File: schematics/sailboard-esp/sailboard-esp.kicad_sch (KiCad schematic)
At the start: 14 parts

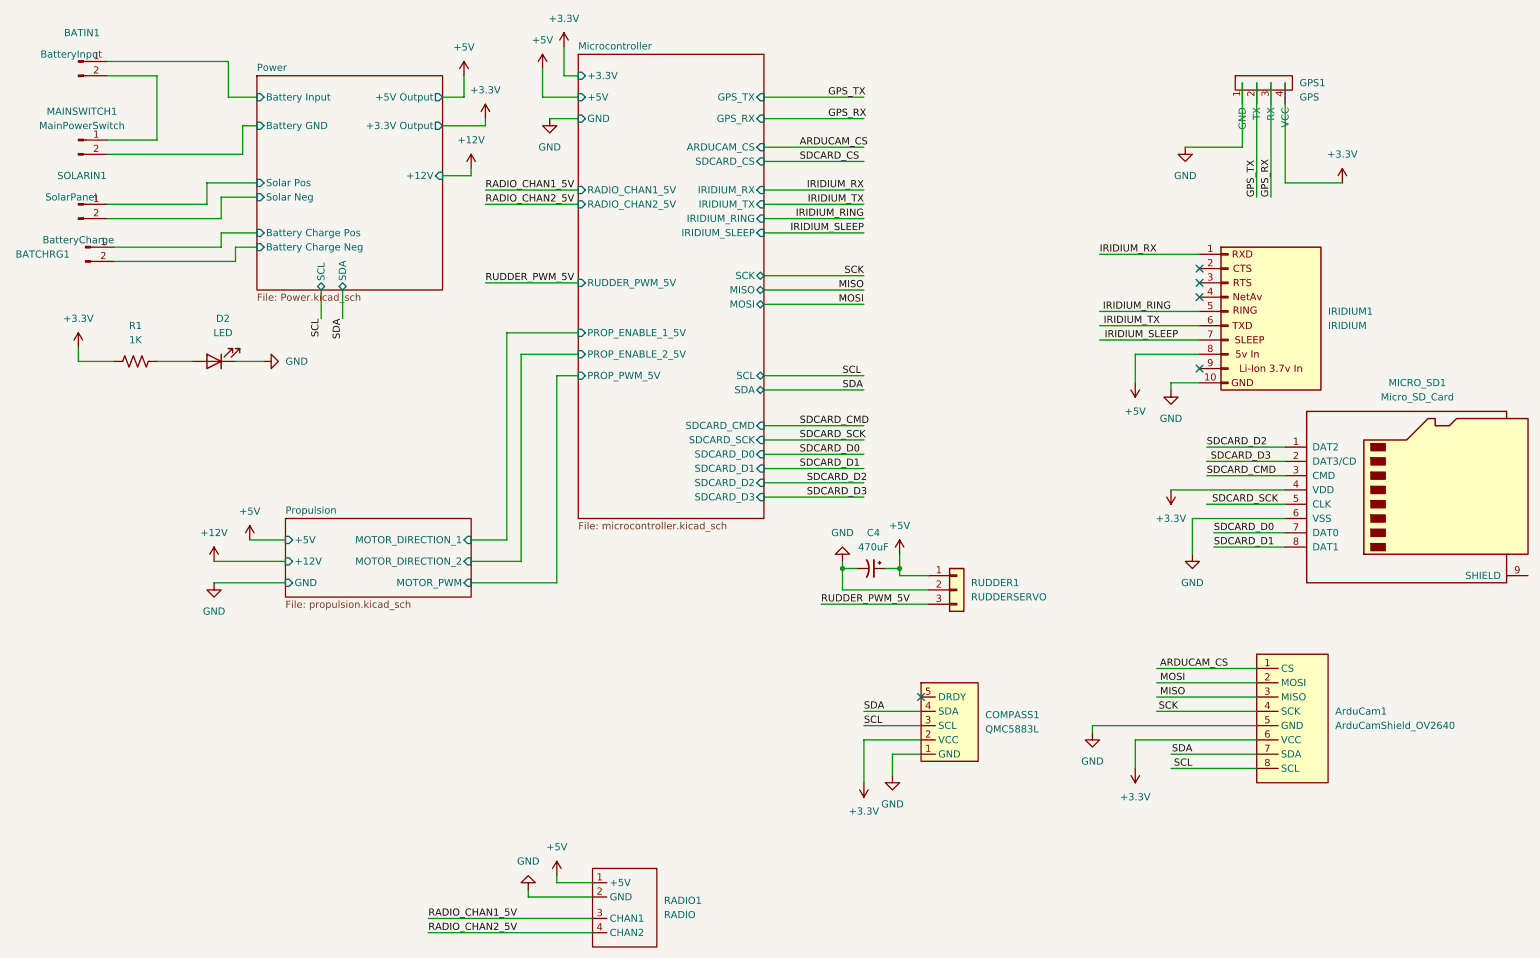
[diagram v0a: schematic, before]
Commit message: v1.3.
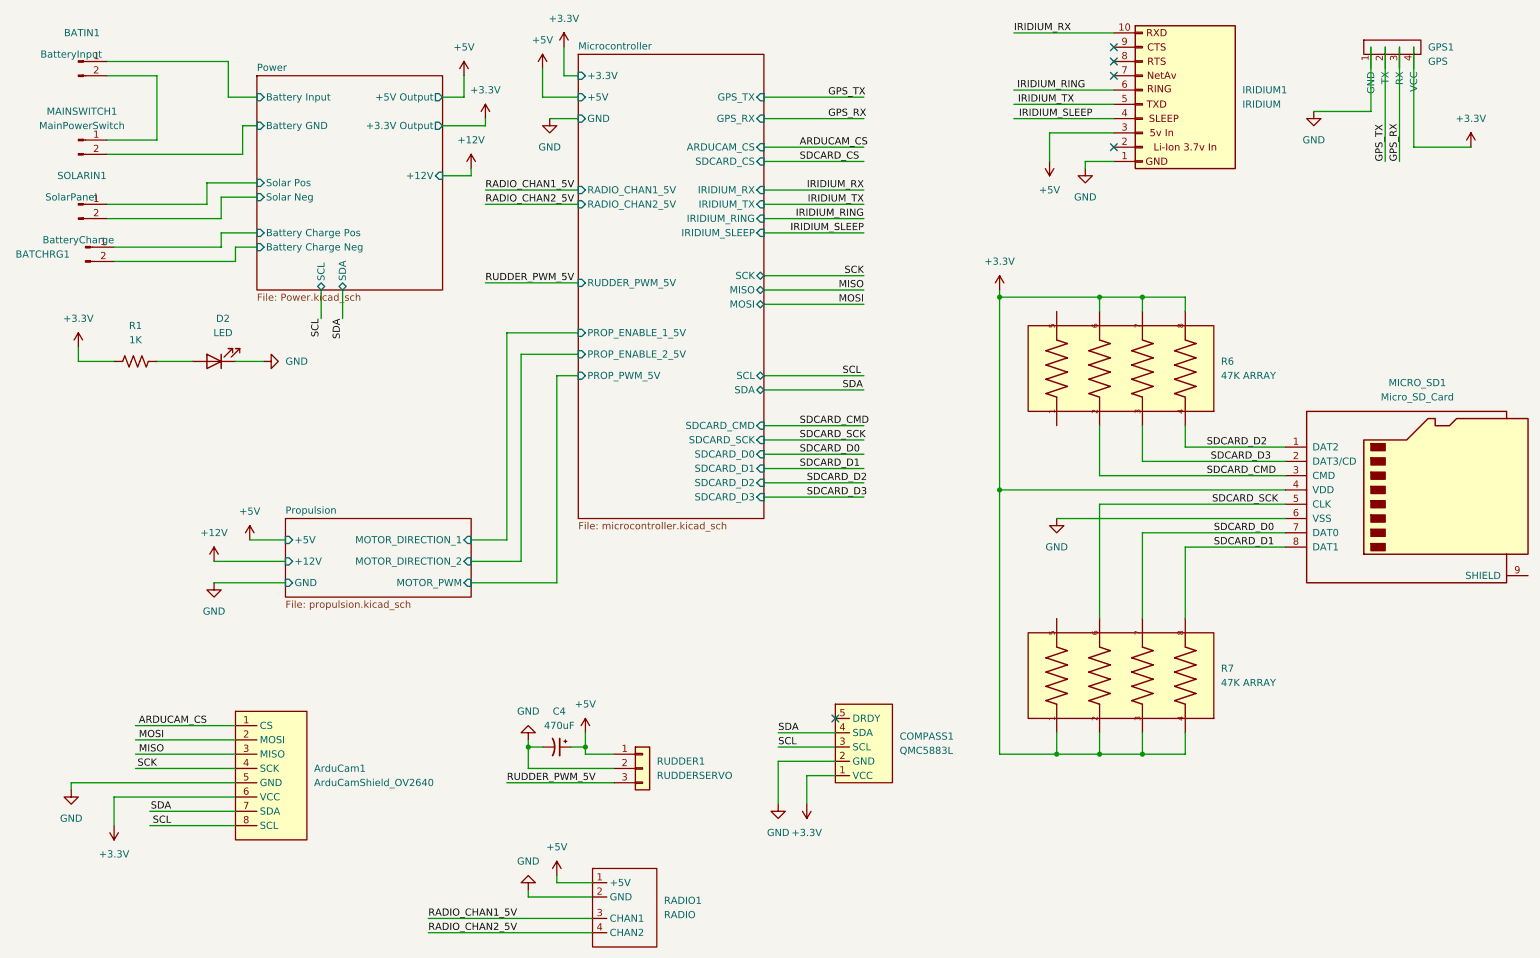
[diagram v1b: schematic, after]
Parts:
- added R6, R7: 47K ARRAY, RESCAXE80P320X160X70-8N, symbol YC164-JR-0747KL:YC164-JR-0747KL
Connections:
- net +3.3V: now also COMPASS1.1 (VCC), R6.6, R6.7, R6.8, R7.1, R7.2, R7.3, R7.4; no longer COMPASS1.2 (VCC)
- net +5V: now also IRIDIUM1.3 (5V); no longer IRIDIUM1.8 (5V)
- net GND: now also COMPASS1.2 (GND), IRIDIUM1.1 (GND); no longer COMPASS1.1 (GND), IRIDIUM1.10 (GND)
- net IRIDIUM_RING: now also IRIDIUM1.6 (RING); no longer IRIDIUM1.5 (RING)
- net IRIDIUM_RX: now also IRIDIUM1.10 (RXD); no longer IRIDIUM1.1 (RXD)
- net IRIDIUM_SLEEP: now also IRIDIUM1.4 (SLEEP); no longer IRIDIUM1.7 (SLEEP)
- net IRIDIUM_TX: now also IRIDIUM1.5 (TXD); no longer IRIDIUM1.6 (TXD)
- net SDCARD_CMD: now also R6.2
- net SDCARD_D0: now also R7.7
- net SDCARD_D1: now also R7.8
- net SDCARD_D2: now also R6.4
- net SDCARD_D3: now also R6.3
- net SDCARD_SCK: now also R7.6
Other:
- moved on the sheet: ArduCam1, C4, COMPASS1, GPS1, IRIDIUM1, RUDDER1
